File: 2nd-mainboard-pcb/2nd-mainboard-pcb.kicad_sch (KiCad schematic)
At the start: 19 parts, among them J1 USB_C_Receptacle, J16 Power, SW1 SW_DIP_x01, U2 FT232RL

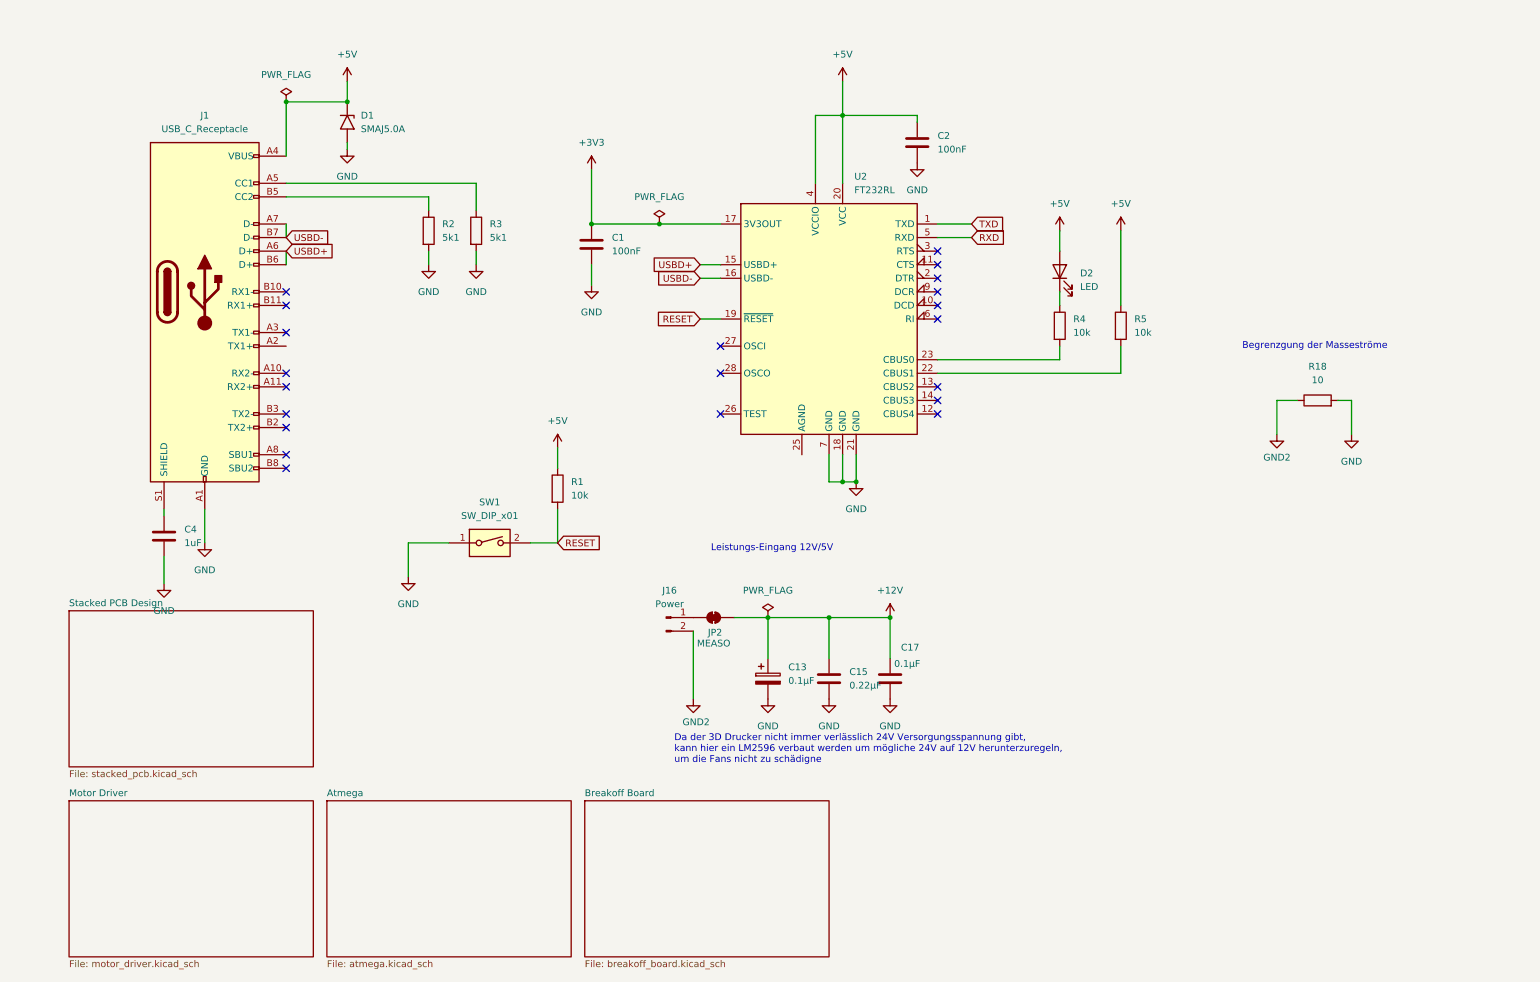
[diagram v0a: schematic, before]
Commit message: verpolungsschutz und powerin
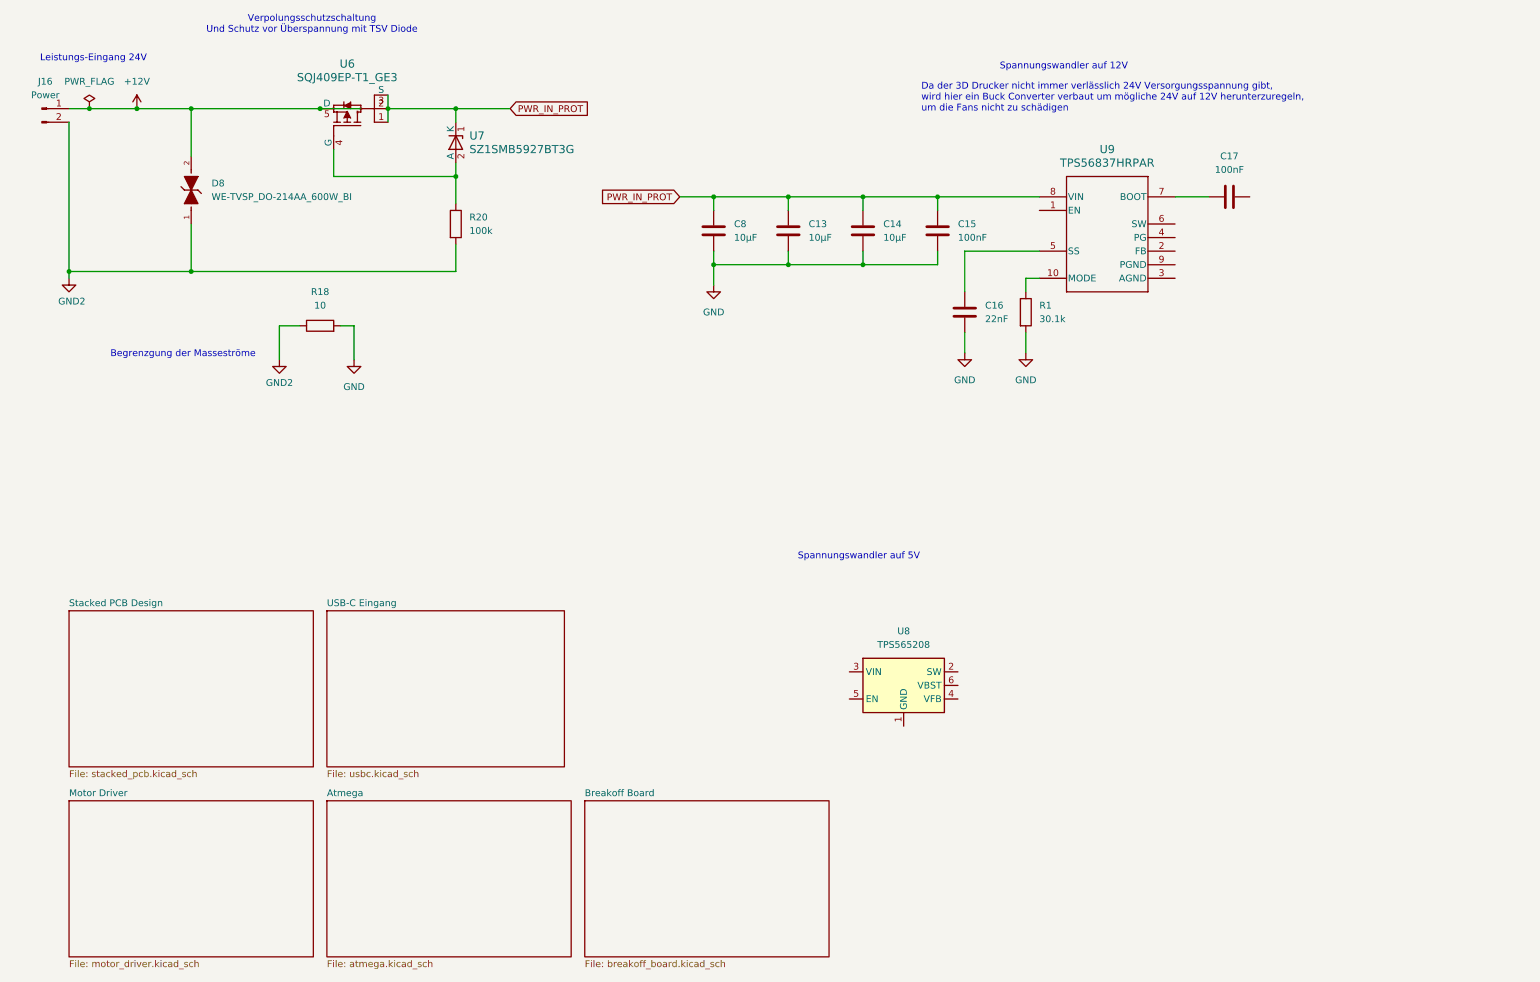
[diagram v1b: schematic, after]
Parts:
- removed C1, C2: 100nF, symbol Device:C
- removed C13: 0.1µF, Capacitor_SMD:CP_Elec_5x3, symbol Device:C_Polarized
- removed C4: 1uF, symbol Device:C
- removed D1: SMAJ5.0A, Diode_SMD:D_SMA, symbol Diode:SMAJ5.0A
- removed D2: LED, symbol Device:LED
- removed J1: USB_C_Receptacle, Connector_USB:USB_C_Receptacle_GCT_USB4085, symbol Connector:USB_C_Receptacle
- removed JP2: MEASO, Jumper:SolderJumper-2_P1.3mm_Bridged_Pad1.0x1.5mm, symbol Jumper:SolderJumper_2_Bridged
- removed R2, R3: 5k1, symbol Device:R
- removed R4, R5: 10k, symbol Device:R
- removed SW1: SW_DIP_x01, Button_Switch_SMD:SW_SPST_EVQQ2, symbol Switch:SW_DIP_x01
- removed U2: FT232RL, Package_SO:SSOP-28_5.3x10.2mm_P0.65mm, symbol Interface_USB:FT232RL
- added C13, C14, C8: 10µF, symbol Device:C
- added C16: 22nF, symbol Device:C
- added D8: WE-TVSP_DO-214AA_600W_BI, WE-TVSP_DO-214AA_600W_BI:WE-TVSP_DO-214AA_BIDIRECTIONAL, symbol Imported_Component_Symbols:WE-TVSP_DO-214AA_600W_BI
- added R20: 100k, symbol Device:R
- added U6: SQJ409EP-T1_GE3, Imported_Component_Footprints:SQJ409EP_T1_GE3, symbol Imported_Component_Symbols:SQJ409EP-T1_GE3
- added U7: SZ1SMB5927BT3G, Imported_Component_Footprints:SZ1SMB5927BT3G, symbol Imported_Component_Symbols:SZ1SMB5927BT3G
- added U8: TPS565208, Package_TO_SOT_SMD:SOT-23-6, symbol Regulator_Switching:TPS565208
- added U9: TPS56837HRPAR, Imported_Component_Footprints:TPS56837HRPAR, symbol Imported_Component_Symbols:TPS56837HRPAR
- C15: value 0.22µF -> 100nF; footprint Capacitor_SMD:C_0402_1005Metric -> (none)
- C17: value 0.1µF -> 100nF; footprint Capacitor_SMD:C_0402_1005Metric -> (none)
- R1: value 10k -> 30.1k
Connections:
- net RESET is gone; now on net GND: R1.2
- net +12V: now also J16.1 (Pin_1), D8.2, U6.5 (D); no longer C15.1, C17.1
- net GND: now also C13.2, C14.2, C16.2, C8.2; no longer C17.2
- net GND2: now also D8.1, R20.2
- net +5V: no longer names the net of R1.1
- net +5V: now also U9.10 (MODE)
- new net: R20.1, U6.4 (G), U7.2 (A)
- new net: C16.1, U9.5 (SS)
- new net: C17.1, U9.7 (BOOT)
- new net PWR_IN_PROT: C13.1, C14.1, C15.1, C8.1, U6.1, U6.2, U6.3 (S), U7.1 (K), U9.8 (VIN)
- no-connect marks 21 -> 0
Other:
- added sheet USB-C Eingang (usbc.kicad_sch)
- note added: "Da der 3D Drucker nicht immer verlässlich 24V Versorgungsspannung gibt, wird hier ein Buck Converter verbaut um mögliche 24V auf 12V herunterzuregeln, um die Fans nicht zu schädigen"
- note added: "Leistungs-Eingang 24V"
- note added: "Spannungswandler auf 12V"
- note added: "Spannungswandler auf 5V"
- note added: "Verpolungsschutzschaltung Und Schutz vor Überspannung mit TSV Diode"
- note removed: "Da der 3D Drucker nicht immer verlässlich 24V Versorgungsspannung gibt, kann hier ein LM2596 verbaut werden um mögliche 24V auf 12V herunterzuregeln, um die Fans nicht zu schädigne"
- note removed: "Leistungs-Eingang 12V/5V"
- moved on the sheet: J16, R18

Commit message: finished stacked design, annotaded
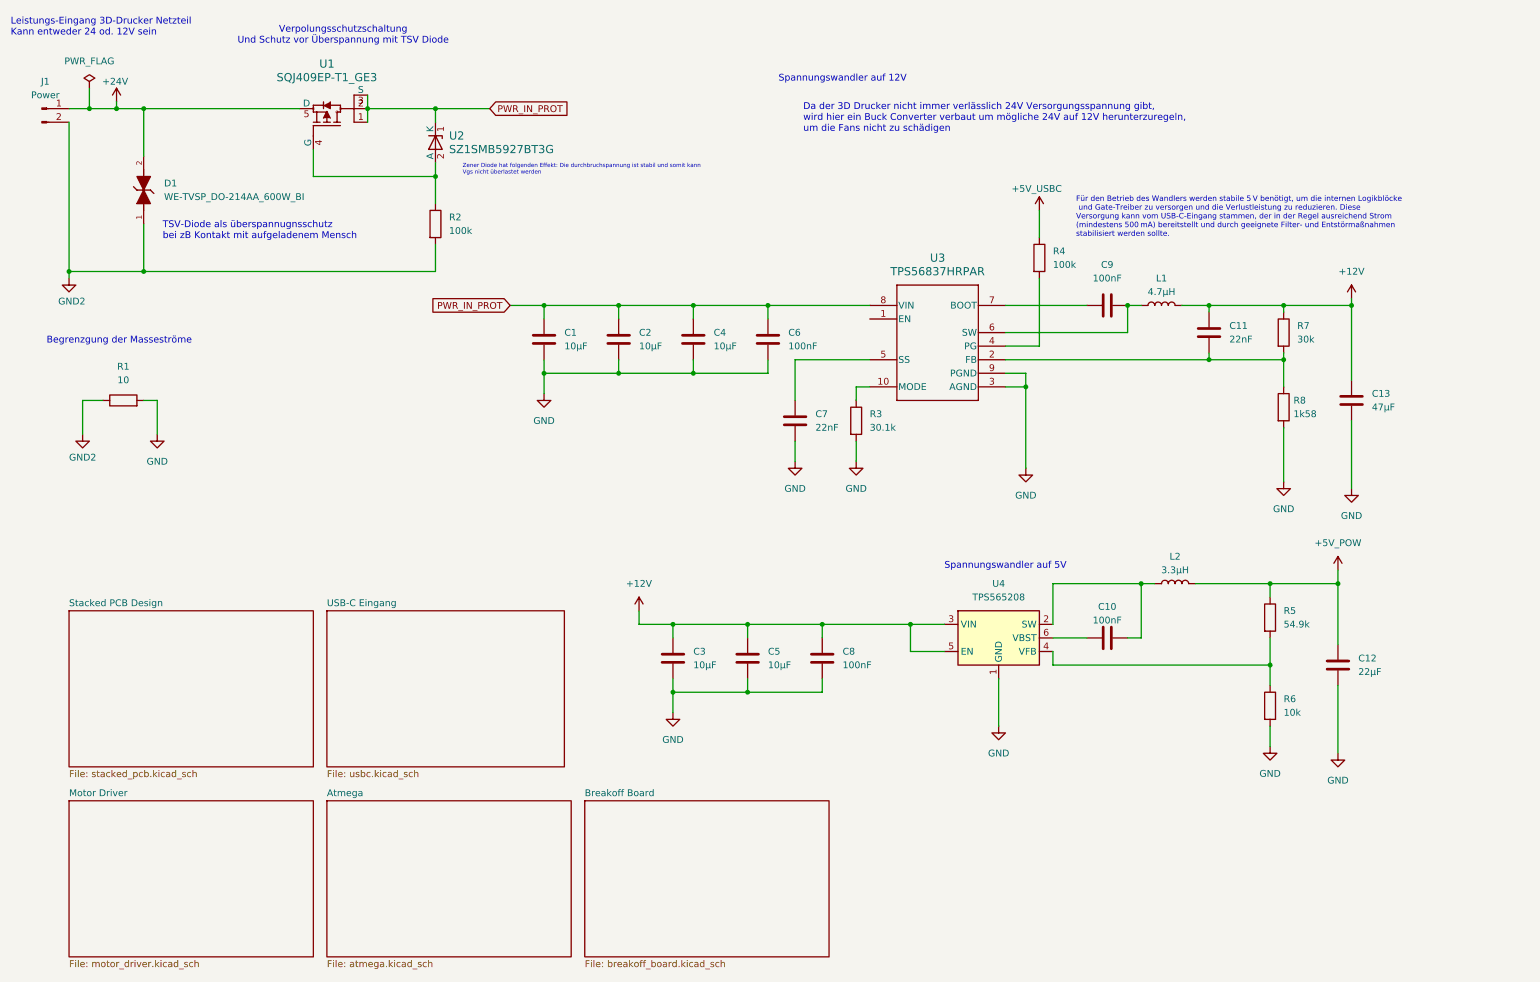
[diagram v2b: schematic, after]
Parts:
- removed C14: 10µF, symbol Device:C
- removed C15, C17: 100nF, symbol Device:C
- removed C16: 22nF, symbol Device:C
- removed R1: 30.1k, symbol Device:R
- removed U9: TPS56837HRPAR, Imported_Component_Footprints:TPS56837HRPAR, symbol Imported_Component_Symbols:TPS56837HRPAR
- added C1, C2, C3, C4, C5: 10µF, symbol Device:C
- added C10, C6, C9: 100nF, symbol Device:C
- added C11, C7: 22nF, symbol Device:C
- added C12: 22µF, symbol Device:C
- added L1: 4.7µH, symbol Device:L
- added L2: 3.3µH, symbol Device:L
- added R3: 30.1k, symbol Device:R
- added R4: 100k, symbol Device:R
- added R5: 54.9k, symbol Device:R
- added R6: 10k, symbol Device:R
- added R7: 30k, symbol Device:R
- added R8: 1k58, symbol Device:R
- added U3: TPS56837HRPAR, Imported_Component_Footprints:TPS56837HRPAR, symbol Imported_Component_Symbols:TPS56837HRPAR
- C13: value 10µF -> 47µF
- C8: value 10µF -> 100nF
- renumbered D8 to D1, J16 to J1, R18 to R1, R20 to R2, U6 to U1, U7 to U2, U8 to U4
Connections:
- net +12V: now also C13.1, C8.1, U4.3 (VIN), U4.5 (EN), C11.1, C3.1, C5.1, L1.2, R7.1; no longer D1.2, J1.1 (Pin_1), U1.5 (D)
- net GND: now also U4.1 (GND), C1.2, C12.2, C2.2, C3.2, C4.2, C5.2, C6.2, C7.2, R3.2, R6.2, R8.2, U3.3 (AGND), U3.9 (PGND)
- net PWR_IN_PROT: now also C1.1, C2.1, C4.1, C6.1, U3.8 (VIN); no longer C13.1, C8.1
- net at U4.2 (SW): now also C10.2, L2.1
- net at U4.4 (VFB): now also R5.2, R6.1
- net at U4.6 (VBST): now also C10.1
- new net: R3.1, U3.10 (MODE)
- new net: C11.2, R7.2, R8.1, U3.2 (FB)
- new net: R4.2, U3.4 (PG)
- new net: C7.1, U3.5 (SS)
- new net: C9.2, L1.1, U3.6 (SW)
- new net: C9.1, U3.7 (BOOT)
- new net +24V: D1.2, J1.1 (Pin_1), U1.5 (D)
- new net +5V_POW: C12.1, L2.2, R5.1
- new net +5V_USBC: R4.1
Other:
- note added: "Für den Betrieb des Wandlers werden stabile 5 V benötigt, um die internen Logikblöcke und Gate-Treiber zu versorgen und die Verlustleistung zu reduzieren. Diese Versorgung kann vom USB‑C‑Eingang stammen, der in der Regel ausreichend Strom (mindestens 500 mA) bereitstellt und durch geeignete Filter- und Entstörmaßnahmen stabilisiert werden sollte."
- note added: "Leistungs-Eingang 3D-Drucker Netzteil Kann entweder 24 od. 12V sein"
- note added: "TSV-Diode als überspannugnsschutz bei zB Kontakt mit aufgeladenem Mensch"
- note added: "Zener Diode hat folgenden Effekt: Die durchbruchspannung ist stabil und somit kann Vgs nicht überlastet werden"
- note removed: "Leistungs-Eingang 24V"
- moved on the sheet: D1, R1, R2, U1, U2, U4
